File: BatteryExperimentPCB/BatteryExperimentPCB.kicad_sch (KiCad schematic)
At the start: 20 parts, among them J1 Screw_Terminal_01x02, J2 Conn_01x10_Pin, J3 Conn_01x10_Pin, U1 BQ25628RYKR, U2 ATtiny3226-M

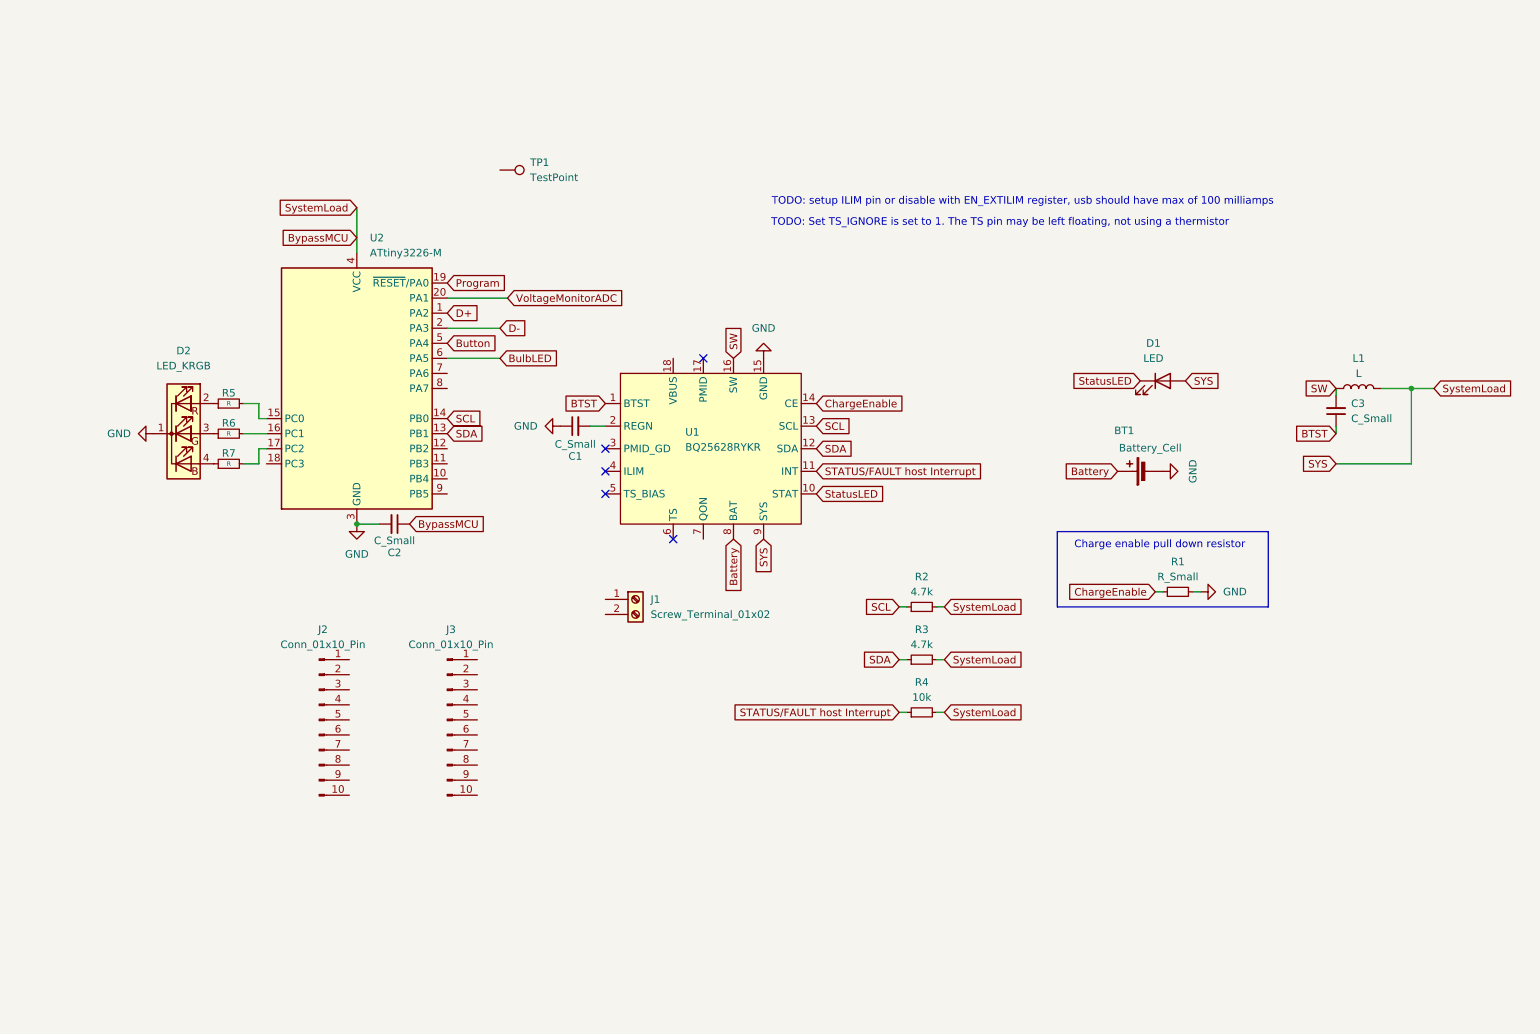
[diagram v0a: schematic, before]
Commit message: wiring lots of stuff up
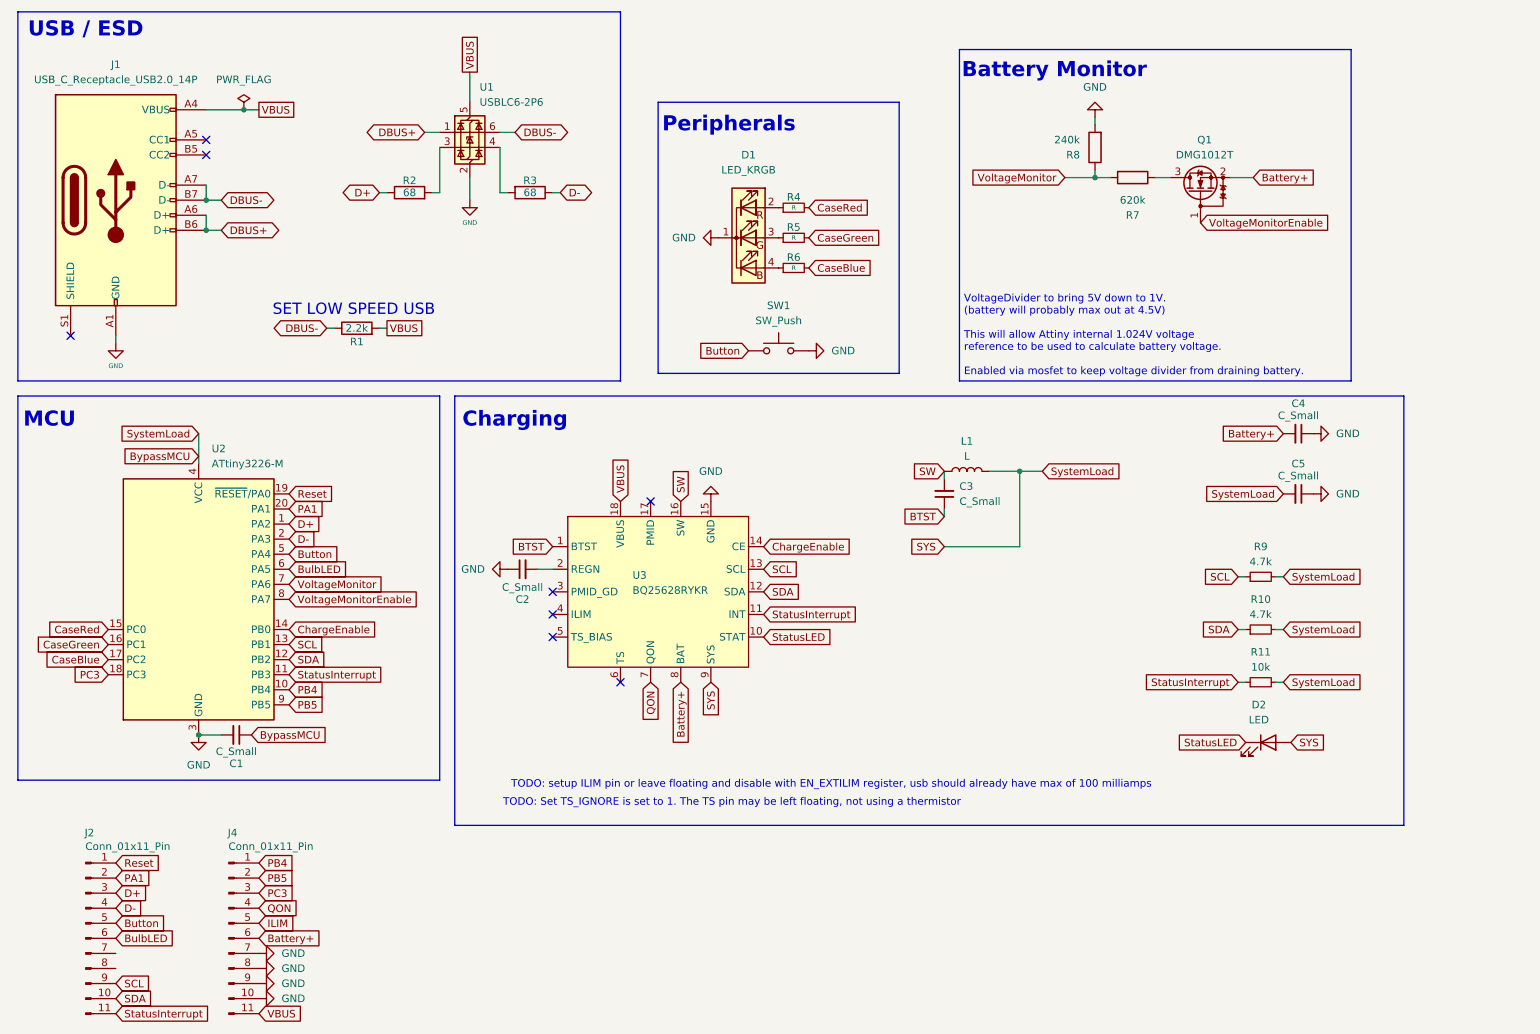
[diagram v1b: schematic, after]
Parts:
- removed BT1: Battery_Cell, symbol Device:Battery_Cell
- removed J1: Screw_Terminal_01x02, symbol Connector:Screw_Terminal_01x02
- removed J2, J3: Conn_01x10_Pin, Connector_PinHeader_2.54mm:PinHeader_1x10_P2.54mm_Vertical, symbol Connector:Conn_01x10_Pin
- removed R1: R_Small, symbol Device:R_Small
- removed TP1: TestPoint, symbol Connector:TestPoint
- added C4, C5: C_Small, symbol Device:C_Small
- added J1: USB_C_Receptacle_USB2.0_14P, Connector_USB:USB_C_Receptacle_G-Switch_GT-USB-7025, symbol Connector:USB_C_Receptacle_USB2.0_14P
- added J2, J4: Conn_01x11_Pin, symbol Connector:Conn_01x11_Pin
- added Q1: DMG1012T, Package_TO_SOT_SMD:SOT-523, symbol Transistor_FET:DMG1012T
- added R1: 2.2k, Resistor_SMD:R_0201_0603Metric, symbol Device:R
- added R2, R3: 68, Resistor_SMD:R_0201_0603Metric, symbol Device:R
- added R7: 620k, symbol Device:R
- added R8: 240k, symbol Device:R
- added SW1: SW_Push, symbol Switch:SW_Push
- added U1: USBLC6-2P6, Package_TO_SOT_SMD:SOT-666, symbol Power_Protection:USBLC6-2P6
- renumbered C2 to C1, C1 to C2, D2 to D1, D1 to D2, R3 to R10, R4 to R11, R5 to R4, R6 to R5, R7 to R6, R2 to R9, U1 to U3
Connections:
- net STATUS/FAULT host Interrupt is gone; now on net StatusInterrupt: R11.1, U3.11 (INT)
- net BulbLED: now also J2.6 (Pin_6)
- net Button: now also J2.5 (Pin_5), SW1.1
- net BypassMCU: now also C5.2
- net ChargeEnable: now also U2.14 (PB0)
- net D+: now also J2.3 (Pin_3), R2.1
- net D-: now also J2.4 (Pin_4), R3.1
- net GND: now also C4.1, C5.1, J1.A1 (GND), J1.A12 (GND), J1.B1 (GND), J1.B12 (GND), J4.10 (Pin_10), J4.7 (Pin_7), J4.8 (Pin_8), J4.9 (Pin_9), R8.2, SW1.2, U1.2 (GND)
- net SCL: now also U2.13 (PB1), J2.9 (Pin_9); no longer U2.14 (PB0)
- net SDA: now also U2.12 (PB2), J2.10 (Pin_10); no longer U2.13 (PB1)
- net VBUS: now reaches U3.18 (VBUS)
- net VBUS: now also J1.A4 (VBUS), J1.A9 (VBUS), J1.B4 (VBUS), J1.B9 (VBUS), J4.11 (Pin_11), R1.2, U1.5 (VBUS)
- net QON: now reaches U3.7 (QON)
- net QON: now also J4.4 (Pin_4)
- net CaseBlue: now reaches R6.2, U2.17 (PC2)
- net CaseRed: now reaches R4.2, U2.15 (PC0)
- net PB4: now reaches U2.10 (PB4)
- net PB4: now also J4.1 (Pin_1)
- net StatusInterrupt: now reaches U2.11 (PB3)
- net StatusInterrupt: now also J2.11 (Pin_11)
- net CaseGreen: now reaches R5.2, U2.16 (PC1)
- net PC3: now reaches U2.18 (PC3)
- net PC3: now also J4.3 (Pin_3)
- net VoltageMonitor: now reaches U2.7 (PA6)
- net VoltageMonitor: now also R7.2, R8.1
- net VoltageMonitorEnable: now reaches U2.8 (PA7)
- net VoltageMonitorEnable: now also Q1.1 (G)
- net PB5: now reaches U2.9 (PB5)
- net PB5: now also J4.2 (Pin_2)
- net Battery renamed Battery+
- net Battery+: now also C4.2, J4.6 (Pin_6), Q1.2 (S)
- net Program renamed Reset
- net Reset: now also J2.1 (Pin_1)
- net VoltageMonitorADC renamed PA1
- net PA1: now also J2.2 (Pin_2)
- new net: Q1.3 (D), R7.1
- new net: R3.2, U1.4 (I/O2)
- new net: R2.2, U1.3 (I/O2)
- new net DBUS+: J1.A6 (D+), J1.B6 (D+), U1.1 (I/O1)
- new net DBUS-: J1.A7 (D-), J1.B7 (D-), R1.1, U1.6 (I/O1)
- new net ILIM: J4.5 (Pin_5)
- no-connect marks 5 -> 8
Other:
- note added: "Battery Monitor"
- note added: "Charging"
- note added: "MCU"
- note added: "Peripherals"
- note added: "SET LOW SPEED USB"
- note added: "TODO: setup ILIM pin or leave floating and disable with EN_EXTILIM register, usb should already have max of 100 milliamps"
- note added: "USB / ESD"
- note added: "VoltageDivider to bring 5V down to 1V. (battery will probably max out at 4.5V) This will allow Attiny internal 1.024V voltage reference to be used to calculate battery voltage. Enabled via mosfet to keep voltage divider from draining battery."
- note removed: "Charge enable pull down resistor"
- note removed: "TODO: setup ILIM pin or disable with EN_EXTILIM register, usb should have max of 100 milliamps"
- moved on the sheet: C1, C2, C3, D1, D2, L1, R10, R11, R4, R5, R6, R9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
